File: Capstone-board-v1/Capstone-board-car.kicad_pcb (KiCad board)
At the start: 2 copper layers, 53.6 x 52.8 mm, 26 parts, among them J1 Pcio Socket 1, J2 Pico Socket 2, J3 Ultra Sonic Sensor, J4 Car, J5 Camera, J6 Gyroscope Sensor, U1 3.3V Voltage Regulator, U2 555 Timer, U3 5V Voltage Regulator 2, U4 5V Voltage Regulator 1

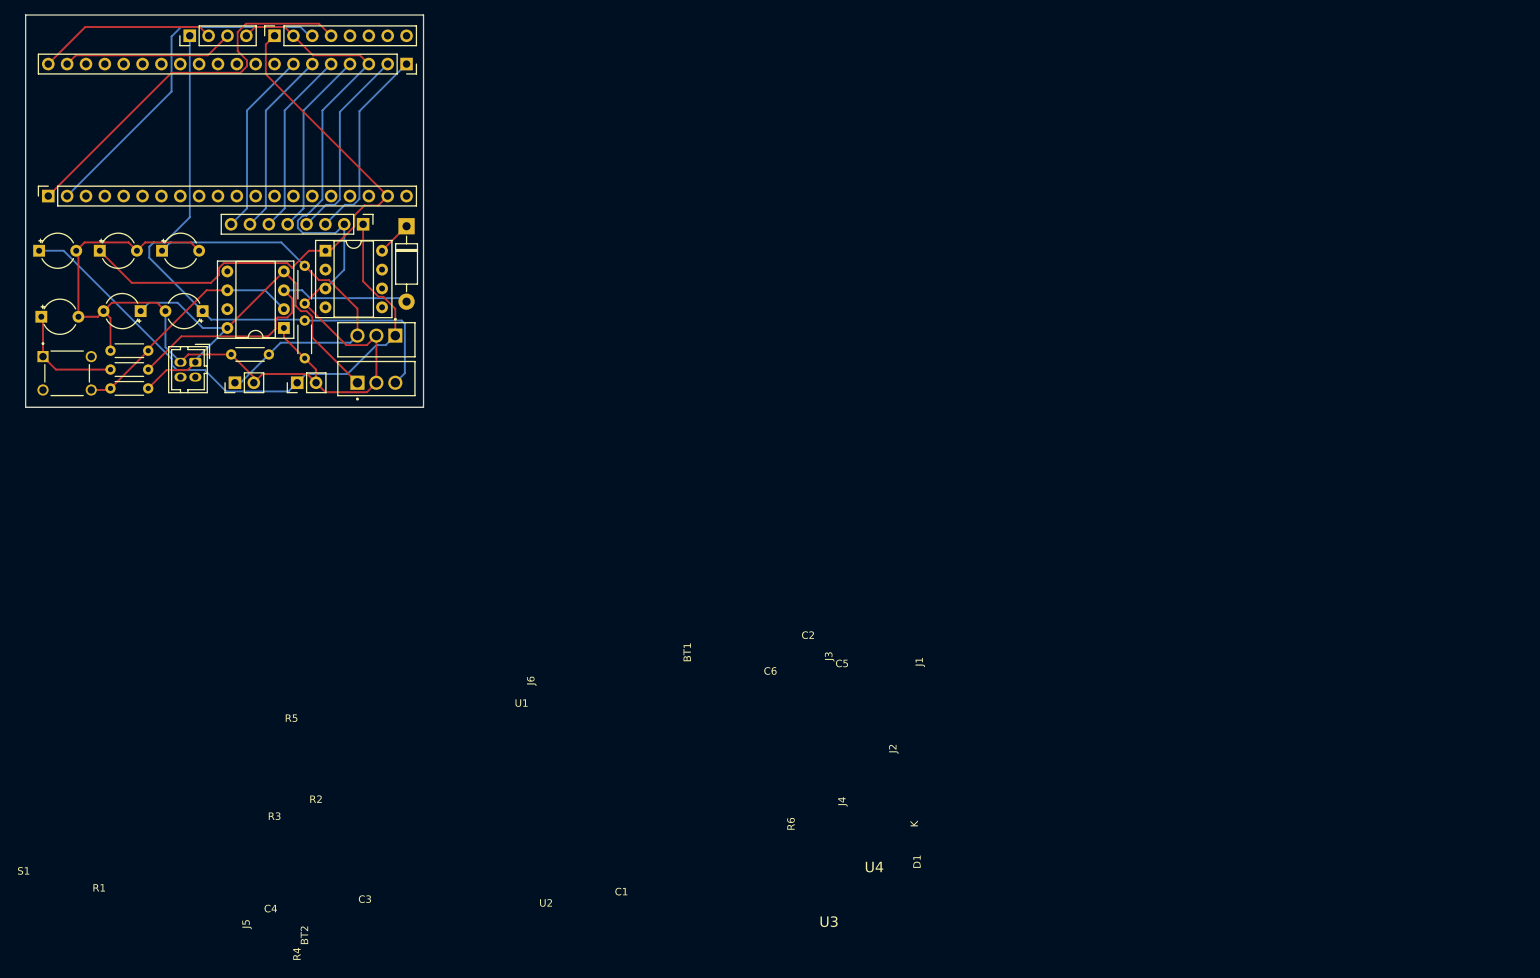
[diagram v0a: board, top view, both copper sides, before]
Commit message: Final traces done
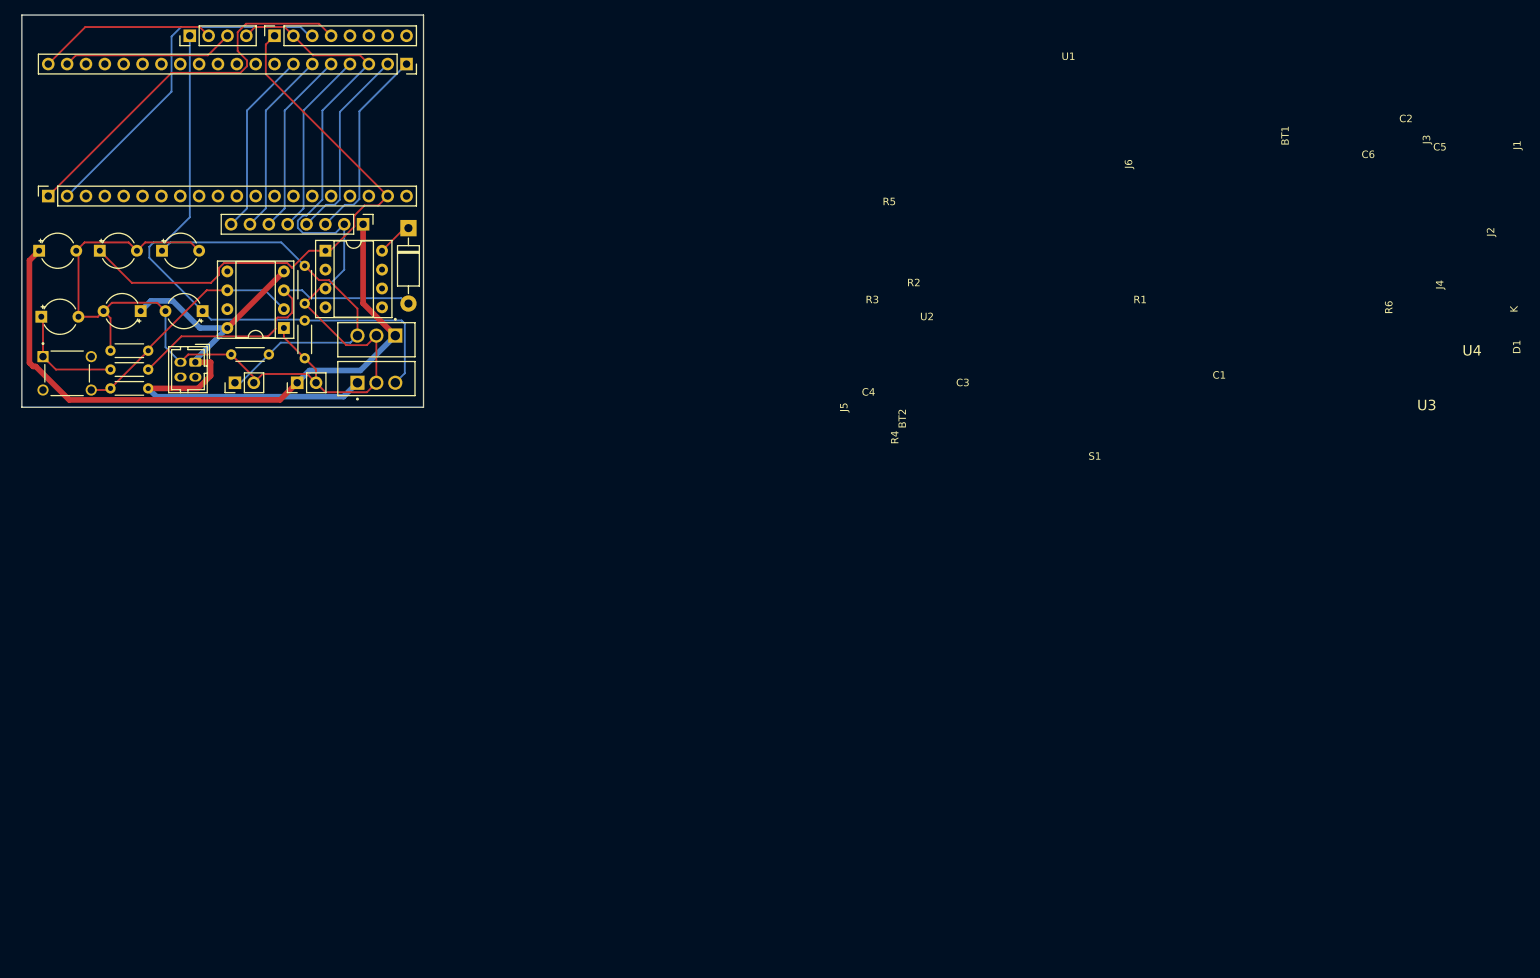
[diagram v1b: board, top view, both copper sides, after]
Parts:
- moved D1 0.36 mm to (87.9, 100.1)
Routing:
- net VCC: track 58.1 -> 73.4 mm
- net VCCQ: track 76.6 -> 87.4 mm
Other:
- board size 53.6 x 52.8 mm -> 54.1 x 52.8 mm
